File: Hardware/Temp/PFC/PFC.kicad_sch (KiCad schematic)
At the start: 33 parts, among them J1 HB9500M-9.5-3P, M1 600V 9.5A, U1 UCC28180D

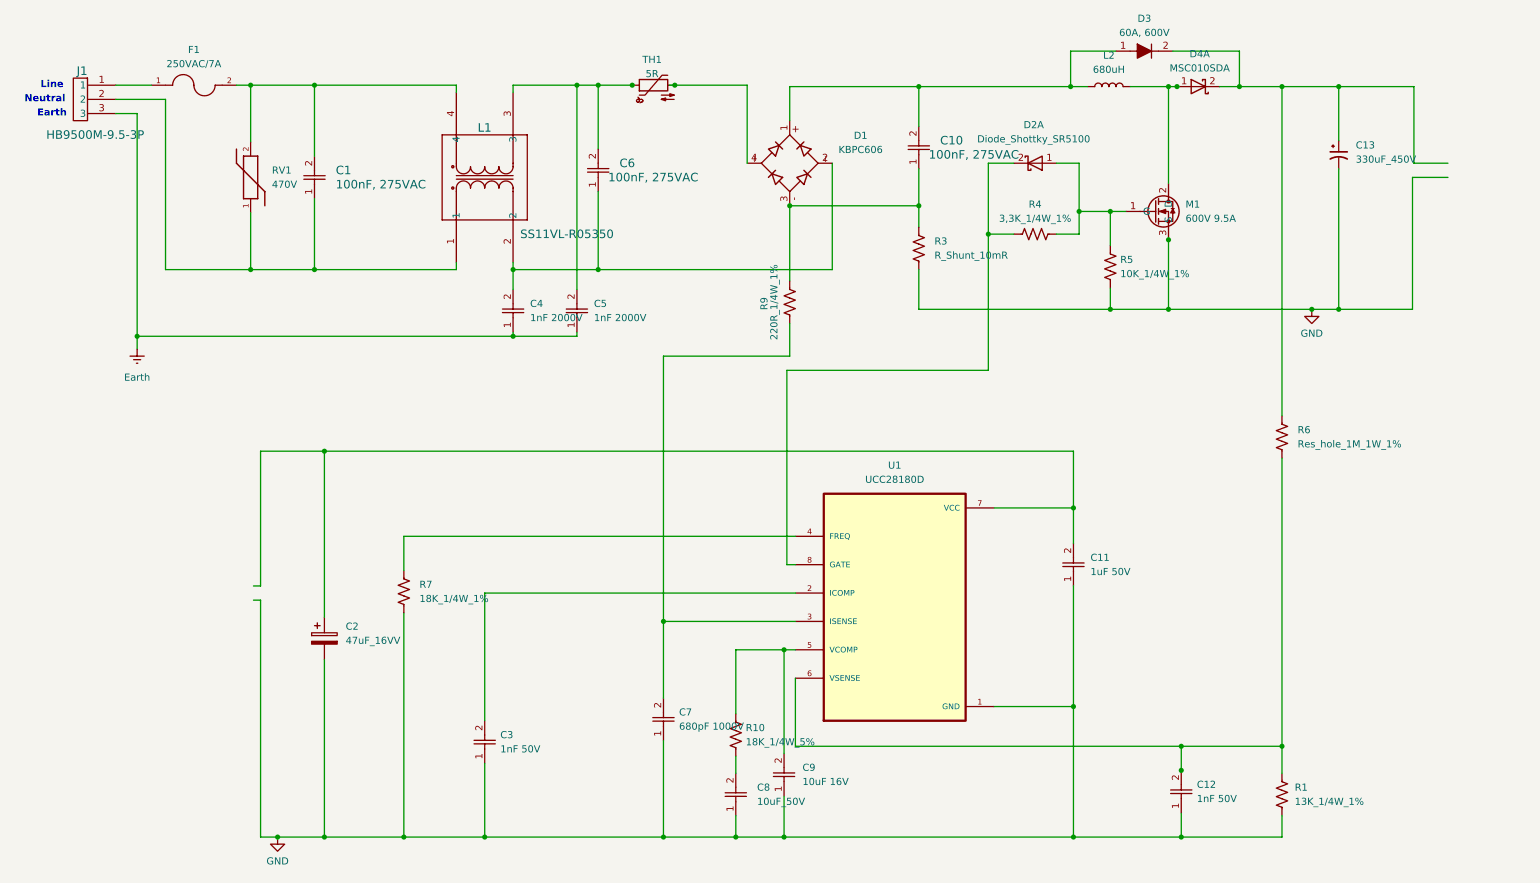
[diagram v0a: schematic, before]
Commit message: completed PFC
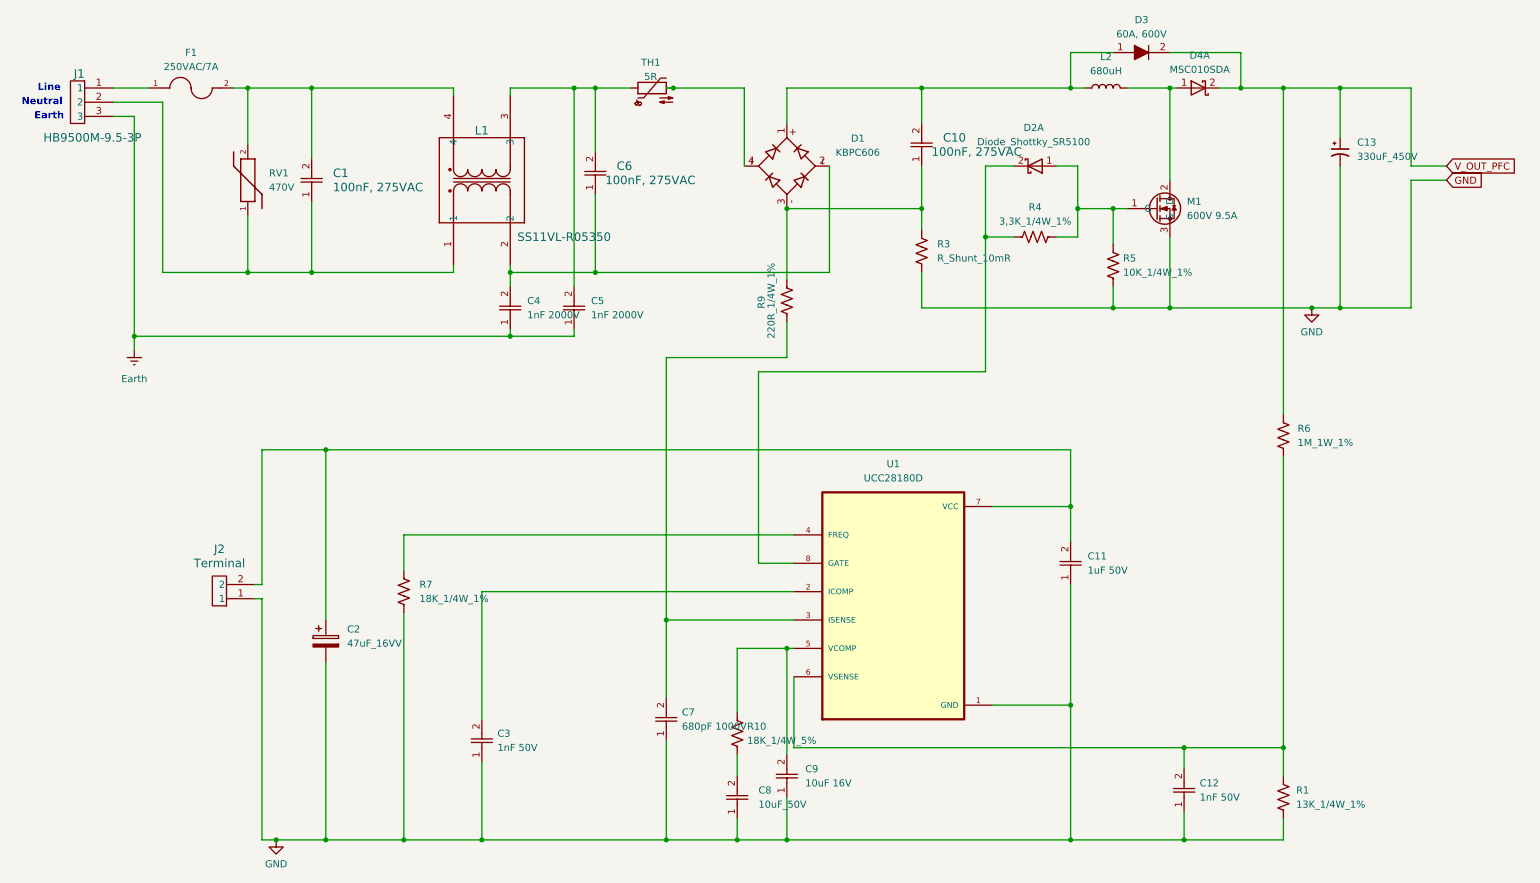
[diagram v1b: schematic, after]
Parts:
- added J2: Terminal, charge_battery_footprint_lib:Terminal, symbol charge_battery_sym_lib:Terminal HB9500-2
- R6: value Res_hole_1M_1W_1% -> 1M_1W_1%
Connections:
- net GND: now also J2.1
- net V_OUT_PFC: now reaches C13.1, D3.2, D4.2 (A), R6.2
- net at C11.2, C2.1, U1.7 (VCC): now also J2.2
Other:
- moved on the sheet: C1, C10, C11, C12, C13, C2, C3, C4, C5, C6, C7, C8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
